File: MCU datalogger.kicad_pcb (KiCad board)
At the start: 2 copper layers, 50.8 x 30.5 mm, 29 parts, among them J1 Conn_01x04_Pin, J2 Conn_01x04_Pin, J3 Conn_01x09_Pin, J4 Conn_02x03_Odd_Even, U1 24LC1025, U2 24LC1025, U3 ATMEGA328P-AU, U4 DS1337S_, Y1 32.768 KHz, Y2 16MHz

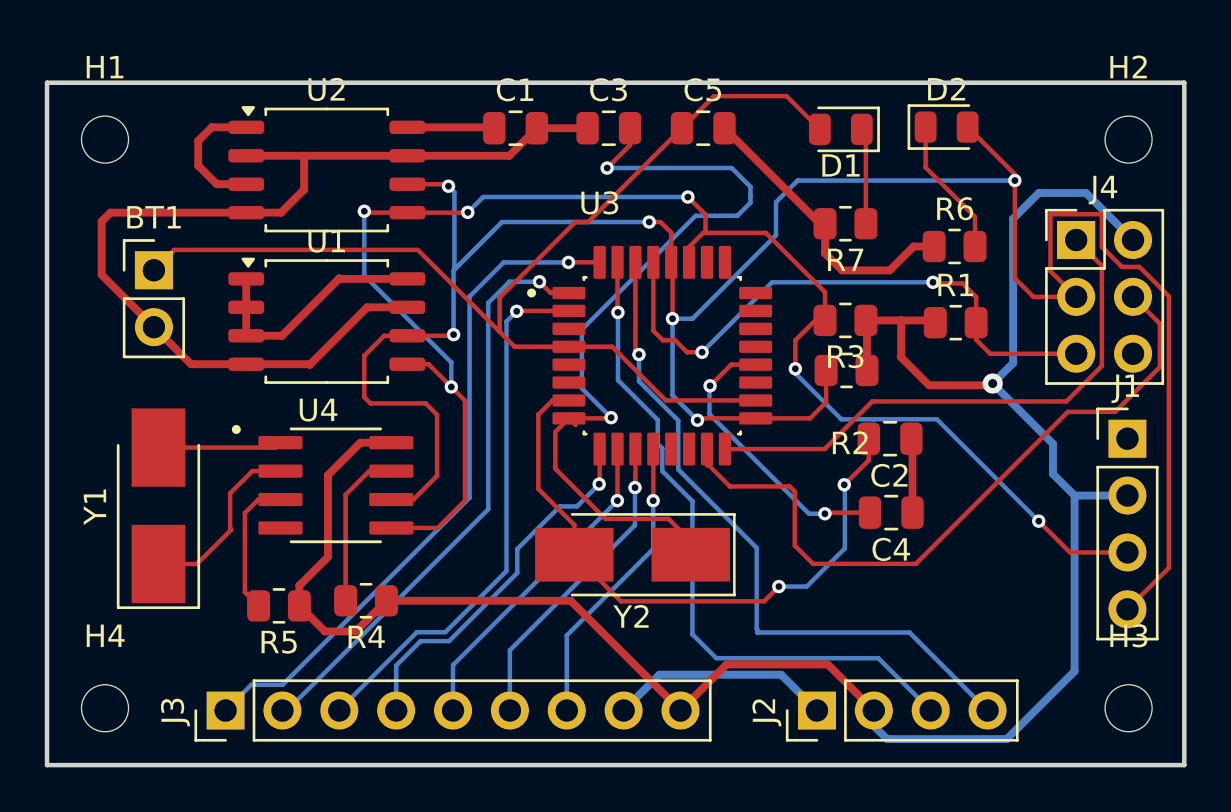
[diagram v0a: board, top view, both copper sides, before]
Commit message: routing complete
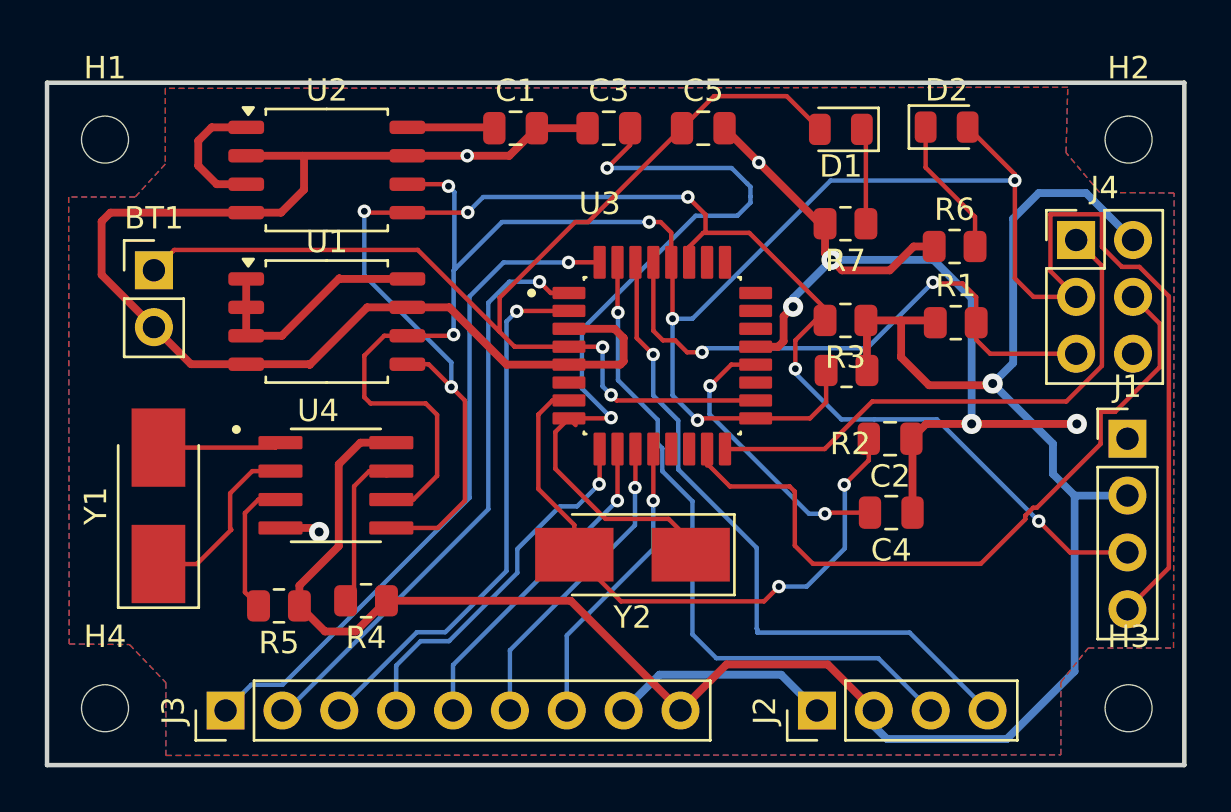
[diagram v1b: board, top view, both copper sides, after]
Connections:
- BT1 pad 1: Net-(BT1-+) -> /VCC
- C5 pad 1: Net-(BT1-+) -> /VCC
- D1 pad 2: Net-(BT1-+) -> /VCC
- U3 pad 18: Net-(BT1-+) -> /VCC
- U3 pad 4: Net-(BT1-+) -> /VCC
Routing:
- net /VCC: track 114.9 -> 166.2 mm, vias 1 -> 3
- net Net-(BT1-+): track 50.2 -> 0.00 mm
- net GND: track 72.2 -> 114.6 mm, vias 0 -> 7
- net /MOSI: track 32.1 -> 33.1 mm
- net /SCK: track 106.7 -> 105.9 mm
- added copper zone on F.Cu, net /VCC
- added copper zone on B.Cu, net GND
